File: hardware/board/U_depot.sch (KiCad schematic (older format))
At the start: 1 part

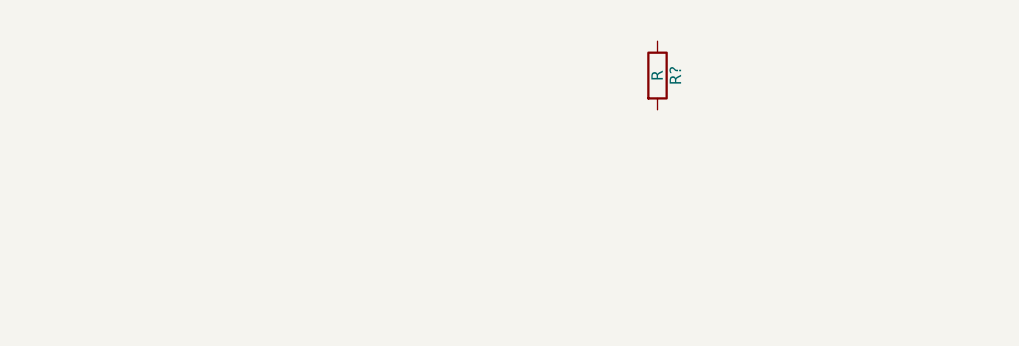
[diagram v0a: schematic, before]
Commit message: added some stuff
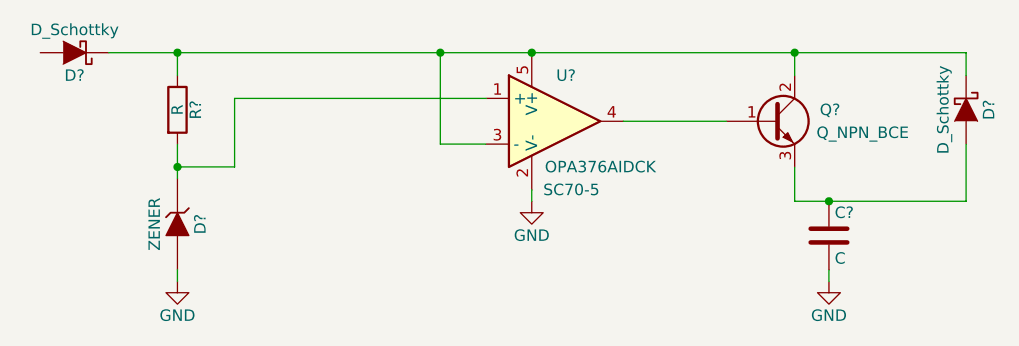
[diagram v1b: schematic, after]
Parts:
- removed R?: R, symbol R
- added C?: C, symbol C
- added D? (x2): D_Schottky, symbol D_Schottky
- added D?: ZENER, symbol ZENER
- added Q?: Q_NPN_BCE, symbol Q_NPN_BCE
- added R?: R, symbol R
- added U?: OPA376AIDCK, SC70-5, symbol OPA376AIDCK
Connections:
- new net: D?.1 (K), D?.1 (K), Q?.2 (C), R?.1, U?.3 (-), U?.5 (V+)
- new net: D?.1 (K), R?.2, U?.1 (+)
- new net: Q?.1 (B), U?.4
- new net: C?.1, D?.2 (A), Q?.3 (E)
- new net GND: C?.2, D?.2 (A), U?.2 (V-)
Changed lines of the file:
@@
 LIBS:contrib
 LIBS:valves
+LIBS:U_depot-cache
 EELAYER 25 0
 EELAYER END
-$Descr A4 11693 8268
+$Descr USLetter 11000 8500
 encoding utf-8
 Sheet 1 1
@@
 $EndDescr
 $Comp
+L D_Schottky D?
+U 1 1 5883CF6D
+P 2750 3700
+F 0 "D?" H 2750 3800 50  0000 C CNN
+F 1 "D_Schottky" H 2750 3600 50  0000 C CNN
+F 2 "" H 2750 3700 50  0000 C CNN
+F 3 "" H 2750 3700 50  0000 C CNN
+	1    2750 3700
+	-1   0    0    1
+$EndComp
+$Comp
 L R R?
-U 1 1 5883CE26
-P 5300 3800
-F 0 "R?" V 5380 3800 50  0000 C CNN
-F 1 "R" V 5300 3800 50  0000 C CNN
-F 2 "" V 5230 3800 50  0000 C CNN
-F 3 "" H 5300 3800 50  0000 C CNN
-	1    5300 3800
+U 1 1 5883CFC8
+P 3200 3950
+F 0 "R?" V 3280 3950 50  0000 C CNN
+F 1 "R" V 3200 3950 50  0000 C CNN
+F 2 "" V 3130 3950 50  0000 C CNN
+F 3 "" H 3200 3950 50  0000 C CNN
+	1    3200 3950
 	1    0    0    -1
 $EndComp
+$Comp
+L ZENER D?
+U 1 1 5883CFE9
+P 3200 4450
+F 0 "D?" H 3200 4550 50  0000 C CNN
+F 1 "ZENER" H 3200 4350 50  0000 C CNN
+F 2 "" H 3200 4450 50  0000 C CNN
+F 3 "" H 3200 4450 50  0000 C CNN
+	1    3200 4450
+	0    1    1    0
+$EndComp
+$Comp
+L GND #PWR?
+U 1 1 5883D03A
+P 3200 4700
+F 0 "#PWR?" H 3200 4450 50  0001 C CNN
+F 1 "GND" H 3200 4550 50  0000 C CNN
+F 2 "" H 3200 4700 50  0000 C CNN
+F 3 "" H 3200 4700 50  0000 C CNN
+	1    3200 4700
+	1    0    0    -1
+$EndComp
+$Comp
+L OPA376AIDCK U?
+U 1 1 5883D06C
+P 4850 4000
+F 0 "U?" H 4900 4200 50  0000 C CNN
+F 1 "OPA376AIDCK" H 5050 3800 50  0000 C CNN
+F 2 "SC70-5" H 4800 3700 50  0000 L CNN
+F 3 "" H 4900 4200 50  0000 C CNN
+	1    4850 4000
+	1    0    0    -1
+$EndComp
+$Comp
+L Q_NPN_BCE Q?
+U 1 1 5883D0DB
+P 5800 4000
+F 0 "Q?" H 6100 4050 50  0000 R CNN
+F 1 "Q_NPN_BCE" H 6400 3950 50  0000 R CNN
+F 2 "" H 6000 4100 50  0000 C CNN
+F 3 "" H 5800 4000 50  0000 C CNN
+	1    5800 4000
+	1    0    0    -1
+$EndComp
+$Comp
+L C C?
+U 1 1 5883D158
+P 6050 4500
+F 0 "C?" H 6075 4600 50  0000 L CNN
+F 1 "C" H 6075 4400 50  0000 L CNN
+F 2 "" H 6088 4350 50  0000 C CNN
+F 3 "" H 6050 4500 50  0000 C CNN
+	1    6050 4500
+	1    0    0    -1
+$EndComp
+$Comp
+L D_Schottky D?
+U 1 1 5883D1D1
+P 6650 3950
+F 0 "D?" H 6650 4050 50  0000 C CNN
+F 1 "D_Schottky" H 6650 3850 50  0000 C CNN
+F 2 "" H 6650 3950 50  0000 C CNN
+F 3 "" H 6650 3950 50  0000 C CNN
+	1    6650 3950
+	0    1    1    0
+$EndComp
+Wire Wire Line
+	5900 4200 5900 4350
+Wire Wire Line
+	5900 4350 6650 4350
+Wire Wire Line
+	6650 4350 6650 4100
+Connection ~ 6050 4350
+$Comp
+L GND #PWR?
+U 1 1 5883D248
+P 6050 4700
+F 0 "#PWR?" H 6050 4450 50  0001 C CNN
+F 1 "GND" H 6050 4550 50  0000 C CNN
+F 2 "" H 6050 4700 50  0000 C CNN
+F 3 "" H 6050 4700 50  0000 C CNN
+	1    6050 4700
+	1    0    0    -1
+$EndComp
+Wire Wire Line
+	6050 4700 6050 4650
+Wire Wire Line
+	2900 3700 6650 3700
+Wire Wire Line
+	5900 3700 5900 3800
+Wire Wire Line
+	6650 3700 6650 3800
+Connection ~ 5900 3700
+Wire Wire Line
+	5150 4000 5600 4000
+Wire Wire Line
+	4550 4100 4350 4100
+Wire Wire Line
+	4350 4100 4350 3700
+Connection ~ 4750 3700
+Wire Wire Line
+	3200 3700 3200 3800
+Connection ~ 4350 3700
+Connection ~ 3200 3700
+Wire Wire Line
+	3200 4250 3200 4100
+Wire Wire Line
+	3200 4700 3200 4650
+Wire Wire Line
+	4550 3900 3450 3900
+Wire Wire Line
+	3450 3900 3450 4200
+Wire Wire Line
+	3450 4200 3200 4200
+Connection ~ 3200 4200
+$Comp
+L GND #PWR?
+U 1 1 5883D63D
+P 4750 4350
+F 0 "#PWR?" H 4750 4100 50  0001 C CNN
+F 1 "GND" H 4750 4200 50  0000 C CNN
+F 2 "" H 4750 4350 50  0000 C CNN
+F 3 "" H 4750 4350 50  0000 C CNN
+	1    4750 4350
+	1    0    0    -1
+$EndComp
+Wire Wire Line
+	4750 4350 4750 4300
 $EndSCHEMATC
